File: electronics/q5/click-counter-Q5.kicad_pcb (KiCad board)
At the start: 2 copper layers, 42 x 54 mm, 93 parts, among them J1 USB-C power and DFU, Q1 Discharge FET, Q2 Charge FET, Q3 Charge enable, Q4 Charge enable hot gate, Q5 COUNT key level shift, SW1 COUNT / POWER, SW2 RESET COUNT / BOOT, SW3 MCU RESET, U1 STM32L072CBT6, U2 Li-ion charger, U3 3.20481V adjustable LDO, U4 Cell protector, U5 Push-pull temperature window, U6 OLED power slew switch, U7 System soft-power latch switch, U8 SPI F-RAM 32KiB

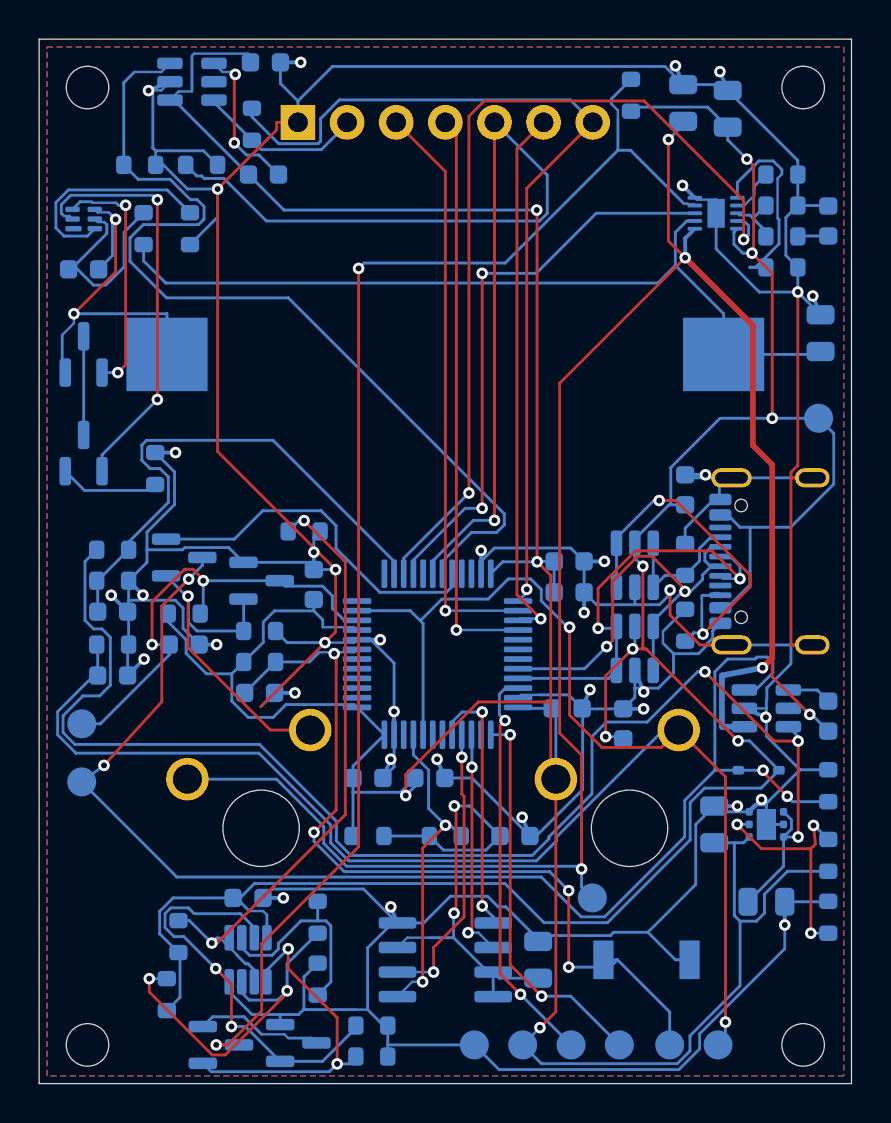
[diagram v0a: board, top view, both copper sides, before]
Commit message: WIP: Q5 design-lock routing iteration snapshot (not verified)
Co-Authored-By: Claude Opus 5.5 <noreply@anthropic.com>
Claude-Session: https://claude.ai/code/session_01UrkzLMrBi6iLPSL5SbMCA7
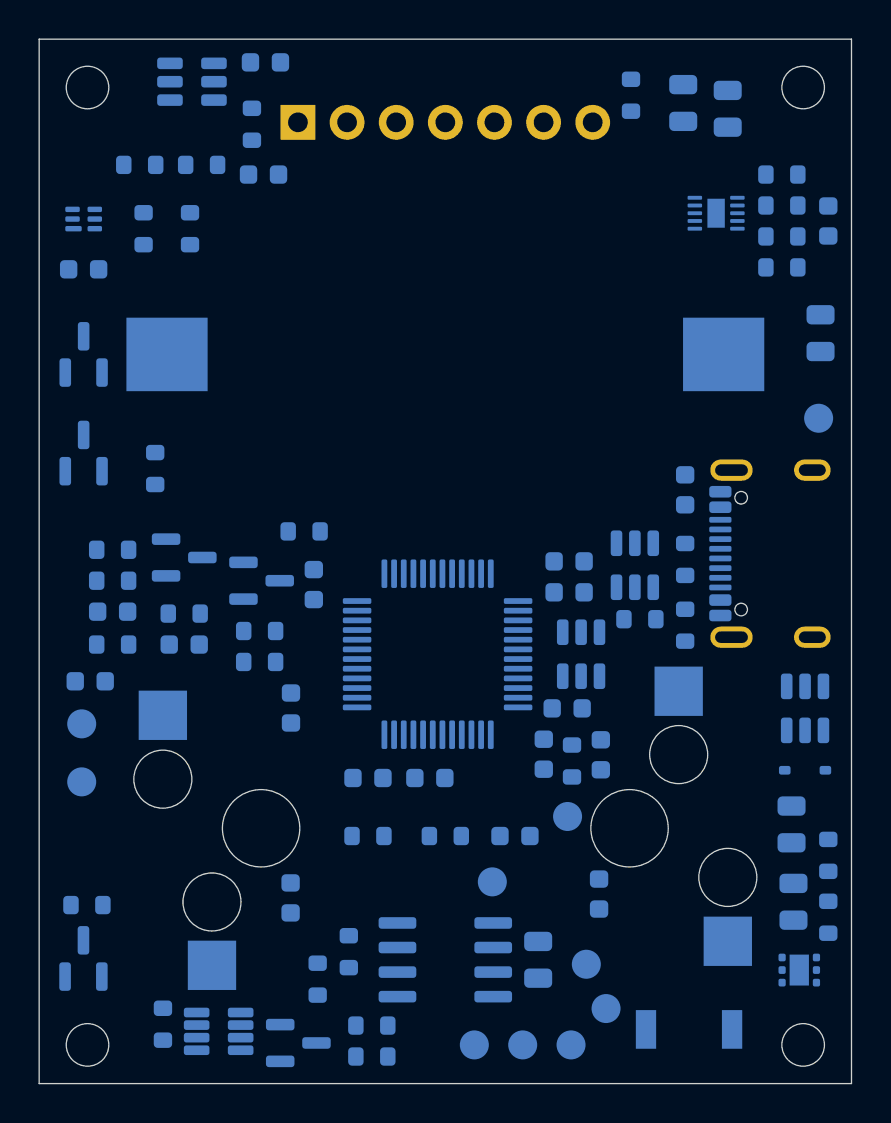
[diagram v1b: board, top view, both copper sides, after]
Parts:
- added C40: 4.7n, CountFidgetQ5:Capacitor_SMD_C_0603_1608Metric, B.Cu at (29.0, 37.0)
- added R38: 100k, CountFidgetQ5:Resistor_SMD_R_0603_1608Metric, B.Cu at (27.6, 37.3)
- SW1, SW2: footprint CountFidgetQ5:HanElectricity_CPG151101D13_MX_Plate -> CountFidgetQ5:SW_Hotswap_Kailh_MX_CPG151101S11; moved to B.Cu
- moved C29 15.0 mm to (28.9, 44.2)
- moved TP12 14.4 mm to (23.4, 43.6)
- moved R35 13.0 mm to (31.1, 30.0), turned to 180 degrees
- moved Q3 8.40 mm to (2.29, 47.5), turned to 90 degrees
- moved U3 7.72 mm to (39.3, 48.1)
- moved R11 6.20 mm to (2.47, 44.8), turned to 180 degrees
- moved TP11 6.00 mm to (28.3, 47.8)
- moved SW1 5.68 mm to (11.5, 40.8), turned to 90 degrees
- moved SW2 5.68 mm to (30.5, 40.8), turned to -90 degrees
- moved R10 4.60 mm to (6.40, 50.9)
- moved TP6 4.40 mm to (27.3, 40.2)
- moved C39 4.40 mm to (26.1, 37.0)
- moved SW3 4.22 mm to (33.6, 51.2)
- moved U5 4.00 mm to (9.28, 51.3), turned to 180 degrees
- moved C6 4.00 mm to (38.9, 40.6)
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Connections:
- D4 pad 1: SYS_ON -> VBUS_WAKE
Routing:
- net GND: track 368.8 -> 0.00 mm, vias 36 -> 0
- net VLOGIC: track 158.4 -> 0.00 mm, vias 4 -> 0
- net VBUS: track 123.4 -> 0.00 mm, vias 7 -> 0
- net SYS: track 103.0 -> 0.00 mm, vias 5 -> 0
- net BOOT_COUNT_RESET: track 92.0 -> 0.00 mm, vias 2 -> 0
- net SYS_LOAD: track 72.9 -> 0.00 mm, vias 3 -> 0
- net SYS_ON: track 71.5 -> 0.00 mm, vias 4 -> 0
- net CE_N: track 70.1 -> 0.00 mm, vias 2 -> 0
- net OLED_RESET_N: track 51.2 -> 0.00 mm, vias 1 -> 0
- net OLED_ENABLE: track 48.1 -> 0.00 mm
- net OLED_CS_N: track 47.1 -> 0.00 mm, vias 1 -> 0
- net CHG_STAT1: track 45.2 -> 0.00 mm, vias 2 -> 0
- net NRST: track 44.1 -> 0.00 mm, vias 4 -> 0
- net CELL_P: track 42.8 -> 0.00 mm
- net TEMP_SENSE: track 32.9 -> 0.00 mm, vias 2 -> 0
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- removed copper zone on B.Cu, net GND
- removed copper zone on F.Cu, net GND
